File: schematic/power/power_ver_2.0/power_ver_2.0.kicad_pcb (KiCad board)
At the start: 2 copper layers, 109.2 x 83.8 mm, 37 parts, among them J1 PWM INPUT, J2 Audio OUTPUT, J3 OUTPUT Power, J4 PWM_power, Q1 RFP12N10L, Q2 RFP12N10L, Q3 RFP12N10L, Q4 RFP12N10L, U1 HIP4082IP

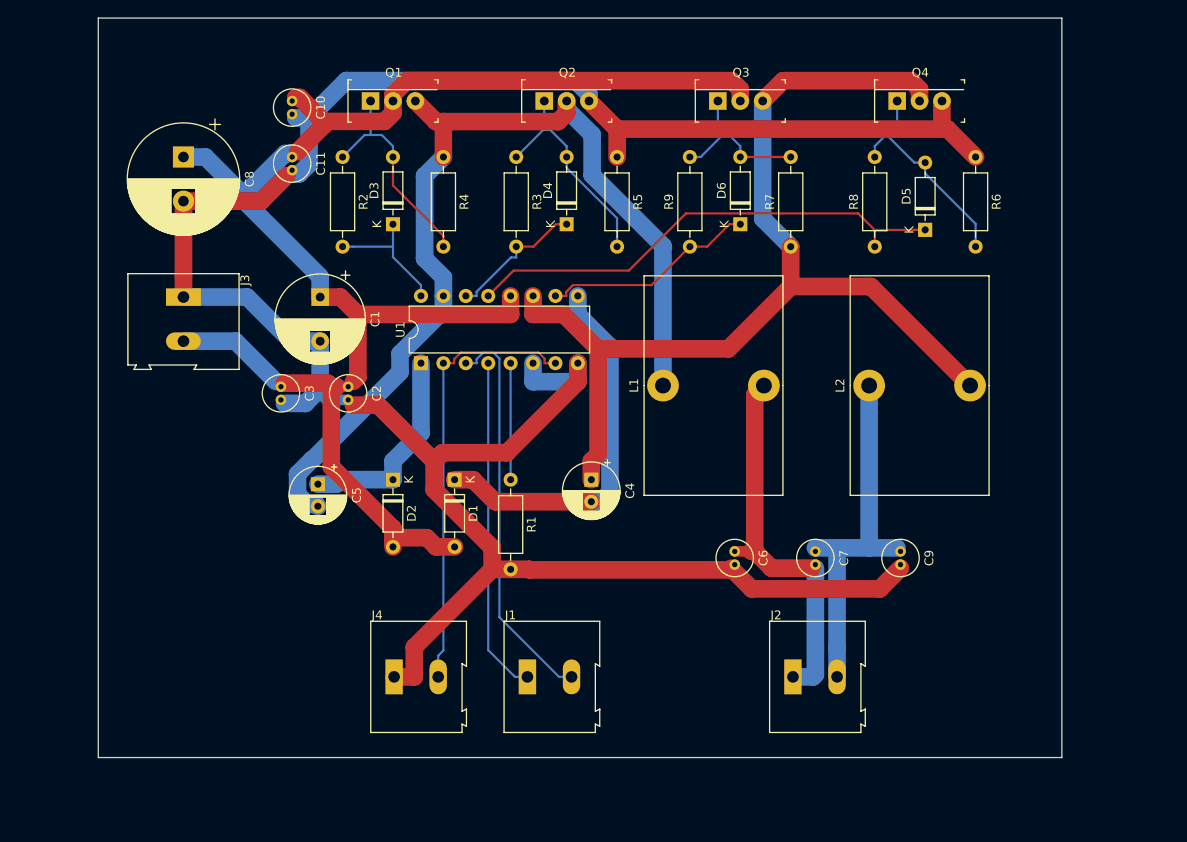
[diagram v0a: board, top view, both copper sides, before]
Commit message: finish pcb trace layout
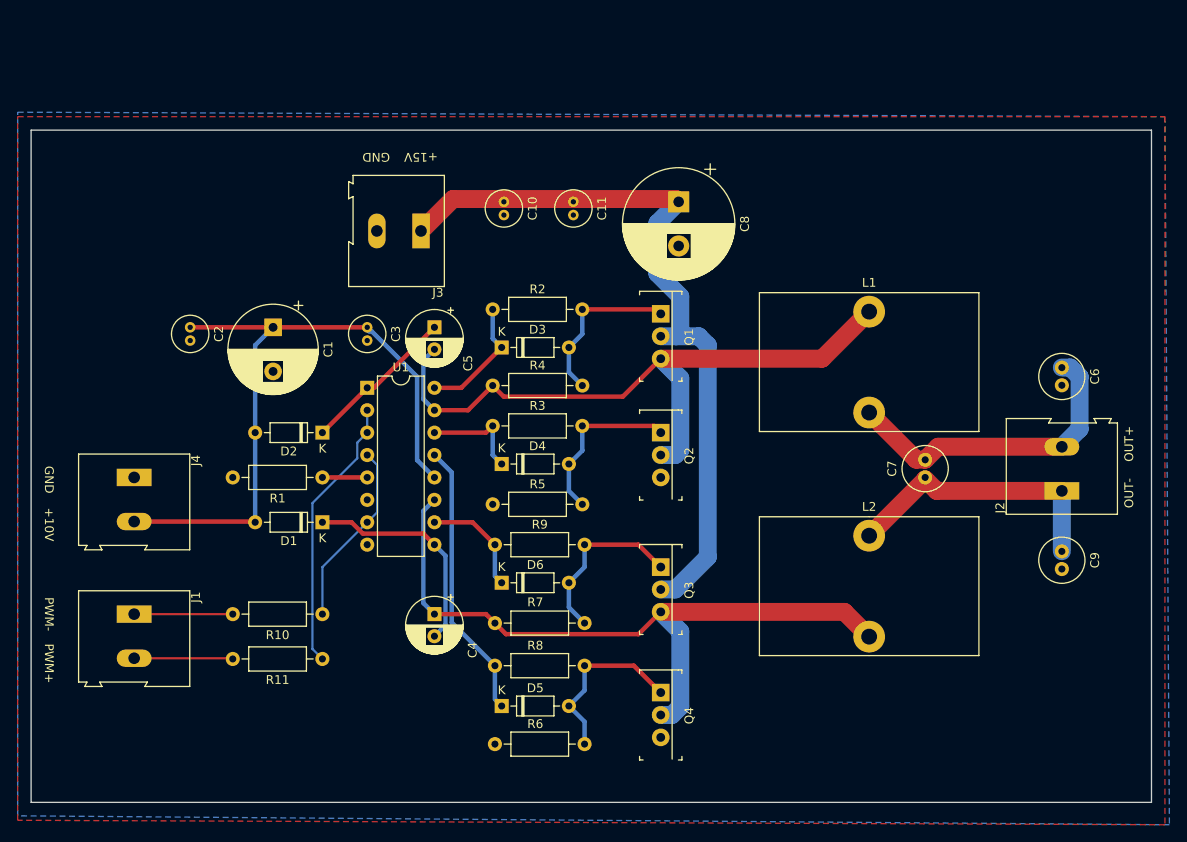
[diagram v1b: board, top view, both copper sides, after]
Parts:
- added R10: 470, Resistor_THT:R_Axial_DIN0207_L6.3mm_D2.5mm_P10.16mm_Horizontal, F.Cu at (109.2, 131.1)
- added R11: 470, Resistor_THT:R_Axial_DIN0207_L6.3mm_D2.5mm_P10.16mm_Horizontal, F.Cu at (109.2, 136.1)
- C6, C7, C9: footprint Capacitor_THT:C_Radial_D4.0mm_H5.0mm_P1.50mm -> Capacitor_THT:C_Radial_D5.0mm_H11.0mm_P2.00mm
- J3: value OUTPUT Power -> Amp_Power
- J4: value PWM_power -> Driver_power
- Q1, Q2, Q3, Q4: value RFP12N10L -> IRF530A
- R2, R3, R8, R9: value R -> 100
- R4, R5, R6, R7: value R -> 10k
- moved R6 86.0 mm to (128.8, 145.8), turned to 0 degrees
- moved D5 72.2 mm to (129.5, 141.5), turned to 0 degrees
- moved Q4 72.2 mm to (147.6, 140.0), turned to 270 degrees
- moved R8 64.1 mm to (128.8, 136.9), turned to 0 degrees
- moved C8 56.4 mm to (149.6, 84.3)
- moved R7 54.3 mm to (128.8, 132.1), turned to 0 degrees
- moved Q3 53.2 mm to (147.6, 125.7), turned to 270 degrees
- moved D6 48.8 mm to (129.5, 127.5), turned to 0 degrees
- moved J1 45.1 mm to (87.9, 131.1), turned to 270 degrees
- moved C6 42.5 mm to (193.0, 103.1)
- moved R5 41.8 mm to (128.5, 118.6), turned to 0 degrees
- moved Q1 40.8 mm to (147.6, 97.0), turned to 270 degrees
- moved R9 40.4 mm to (128.8, 123.2), turned to 0 degrees
- moved Q2 39.8 mm to (147.6, 110.5), turned to 270 degrees
- moved J4 37.1 mm to (87.9, 115.6), turned to 270 degrees
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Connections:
- net Net-(C4-Pad1) renamed /A_HI
- net Net-(C5-Pad2) renamed /B_HI
- net Net-(D3-Pad1) renamed /BHO
- net Net-(D4-Pad1) renamed /BLO
- net Net-(D5-Pad1) renamed /ALO
- net Net-(D6-Pad1) renamed /AHO
- C1 pad 1: +15V -> +10V
- C2 pad 1: +15V -> +10V
- C3 pad 1: +15V -> +10V
- D1 pad 2: +15V -> +10V
- D2 pad 2: +15V -> +10V
- J2 pad 1: Out+ -> Out-
- J2 pad 2: Out- -> Out+
- J3 pad 1: GND -> +15V
- J3 pad 2: +15V -> GND
- J4 pad 2: +5V -> +10V
- U1 pad 12: +15V -> +10V
- U1 pad 2: +5V -> Net-(R11-Pad1)
- U1 pad 3: PWM+ -> Net-(R11-Pad1)
- U1 pad 4: PWM- -> Net-(R10-Pad1)
- U1 pad 7: +5V -> Net-(R10-Pad1)
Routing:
- net GND: track 280.6 -> 0.00 mm
- net +15V: track 176.6 -> 85.0 mm
- net +10V: track 0.00 -> 77.1 mm
- net +5V: track 50.1 -> 0.00 mm
- net /A_HI: track 118.8 -> 80.7 mm
- net /B_HI: track 110.7 -> 76.6 mm
- net PWM+: track 45.2 -> 11.2 mm
- net Net-(R11-Pad1): track 0.00 -> 31.2 mm
- net PWM-: track 38.2 -> 11.2 mm
- net /ALO: track 56.1 -> 31.6 mm
- net Net-(R10-Pad1): track 0.00 -> 21.1 mm
- net Net-(C4-Pad2): track 42.9 -> 25.2 mm
- net /AHO: track 24.6 -> 12.5 mm
- net Out-: track 43.2 -> 31.9 mm
- net Out+: track 44.4 -> 35.9 mm
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- added copper zone on B.Cu, net GND
- added copper zone on F.Cu, net GND
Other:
- board size 109.2 x 83.8 mm -> 127 x 76.2 mm
- board text added: "+10V"
- board text added: "+15V"
- board text added: "GND"
- board text added: "OUT+"
- board text added: "OUT-"
- board text added: "PWM+"
- board text added: "PWM-"
